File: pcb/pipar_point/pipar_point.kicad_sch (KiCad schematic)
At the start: 0 parts

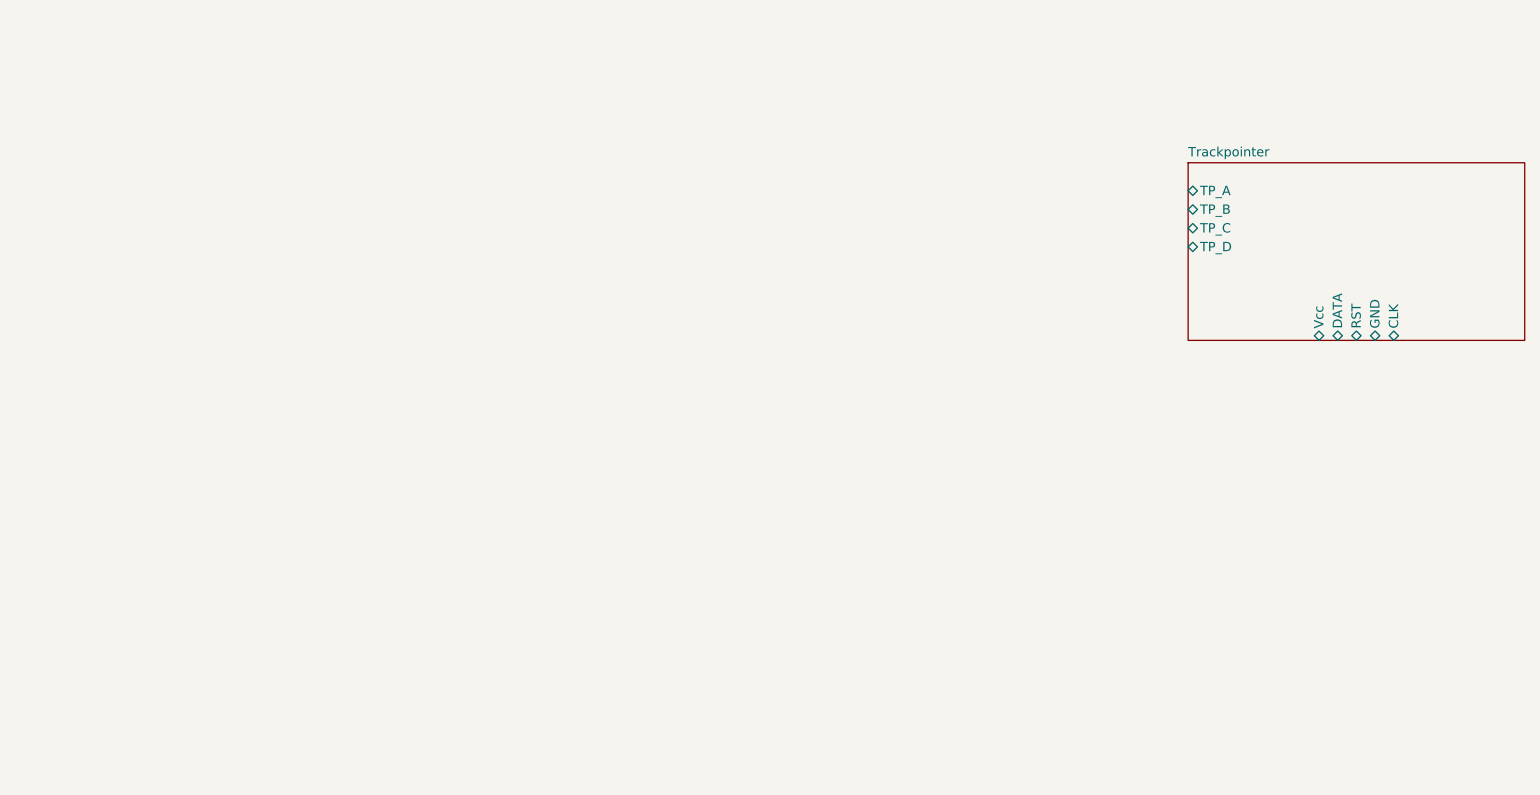
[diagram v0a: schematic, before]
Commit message: more pipar poimt progress
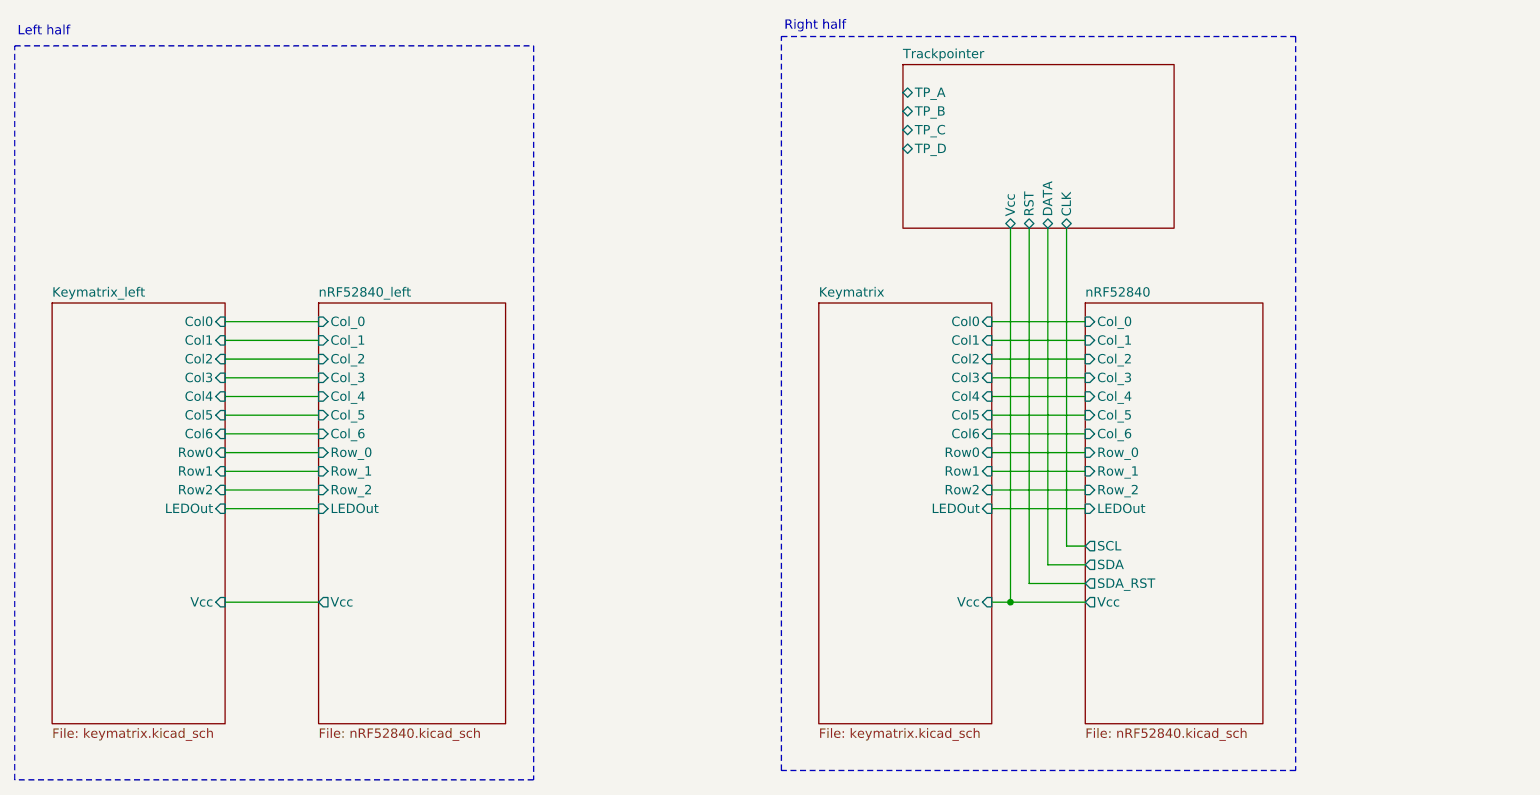
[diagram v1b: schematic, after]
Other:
- added sheet Keymatrix (keymatrix.kicad_sch)
- added sheet Keymatrix_left (keymatrix.kicad_sch)
- added sheet nRF52840 (nRF52840.kicad_sch)
- added sheet nRF52840_left (nRF52840.kicad_sch)
- sheet Trackpointer ports: added none; removed GND
- note added: "Left half"
- note added: "Right half"
